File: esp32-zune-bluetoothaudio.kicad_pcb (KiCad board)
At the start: 2 copper layers, 36 parts, among them J1 Conn_01x06, J2 USB_C_Receptacle_USB2.0, J3 zune connector, Q1 MMBT3904, Q2 MMBT3904, Q3 MMBT3904, Q4 MMBT3904, U1 TPM, U2 ESP32-A1S, U3 AP1117-33

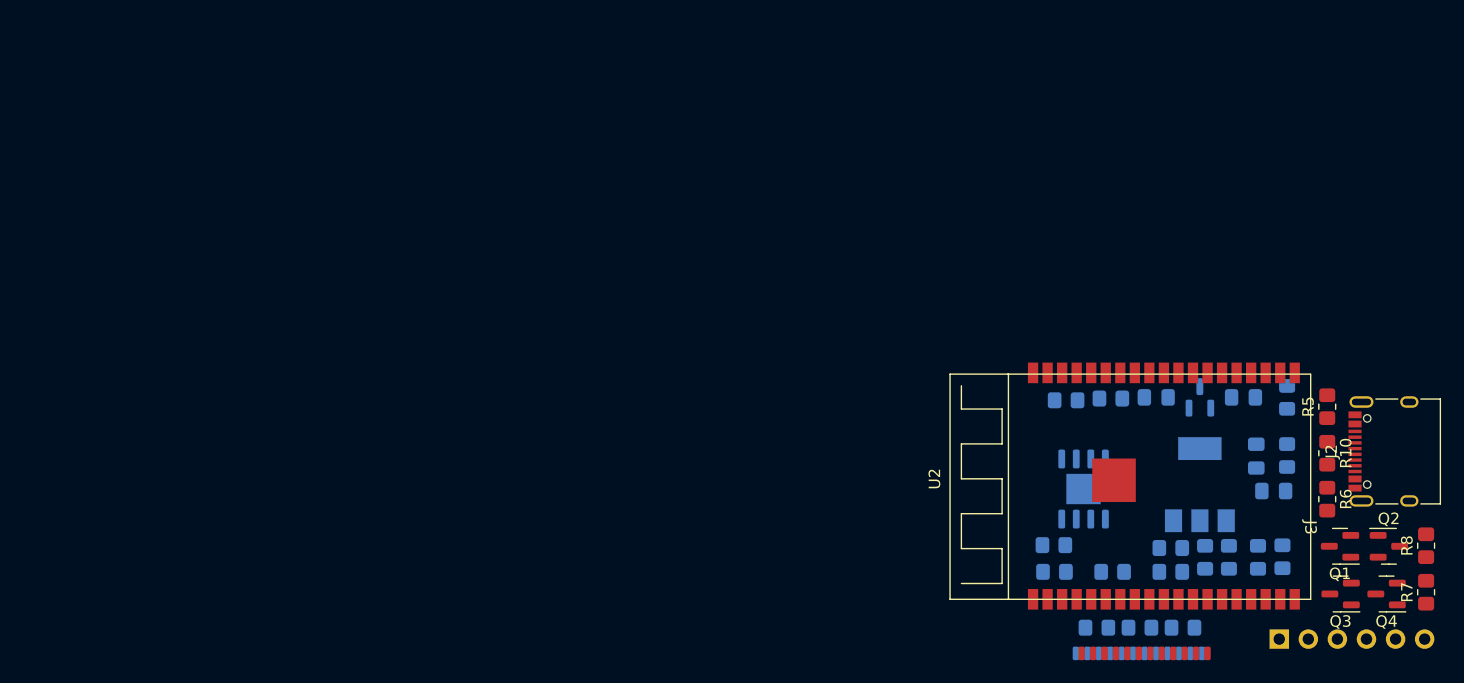
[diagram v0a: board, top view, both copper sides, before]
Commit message: layoutish
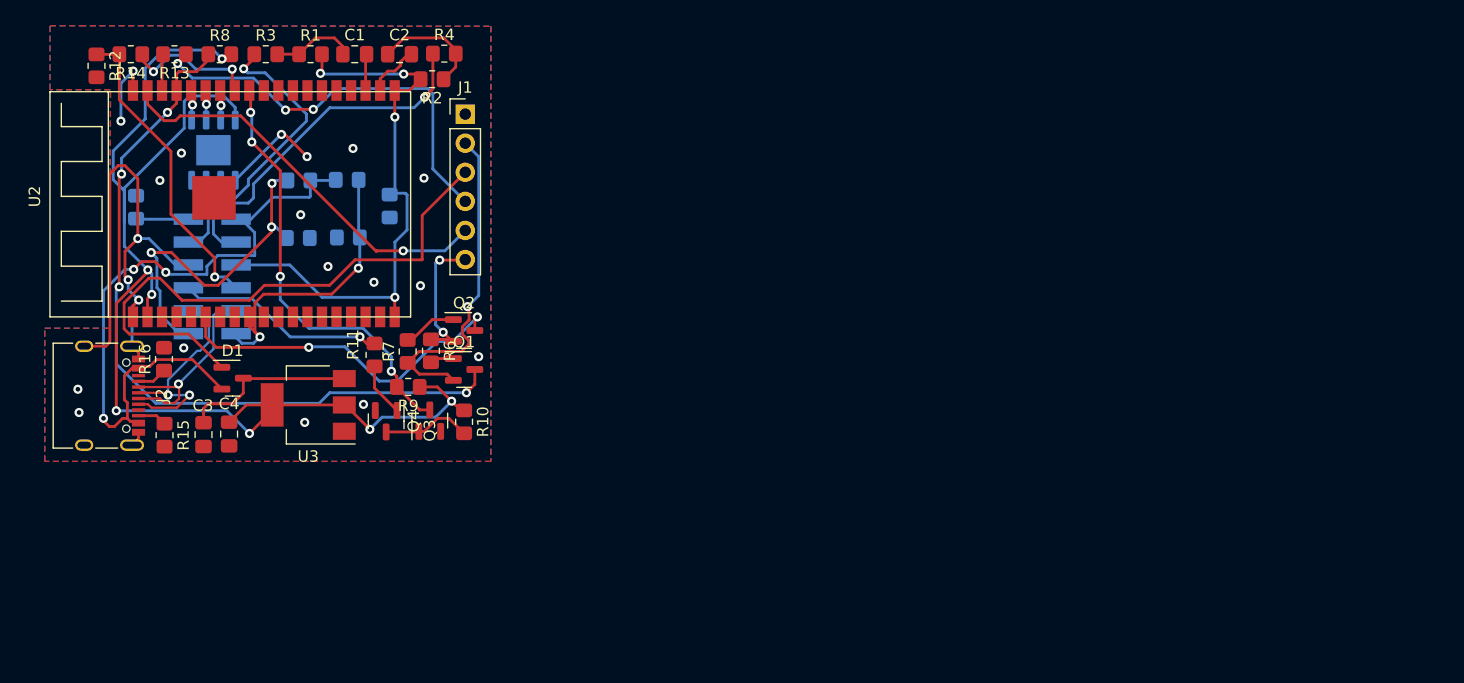
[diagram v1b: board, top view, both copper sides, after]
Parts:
- C1, C2, C3, C4, D1, R1, R11, R12, R13, R14, R15, R16, R2, R3, R4, R9, U3: moved to F.Cu
- J1: footprint Connector_PinSocket_2.54mm:PinSocket_1x06_P2.54mm_Horizontal -> Connector_PinHeader_2.54mm:PinHeader_1x06_P2.54mm_Vertical; moved to F.Cu
- J3: value zune connector -> Zune Passthrough; footprint ZuneConnector:zune-edge-connector -> Connector_PinHeader_2.00mm:PinHeader_2x06_P2.00mm_Vertical_SMD; moved to B.Cu
- R5: moved to B.Cu
- moved R8 113.8 mm to (120.1, 81.8), turned to 0 degrees
- moved J2 113.7 mm to (109.4, 111.6), turned to -90 degrees
- moved R14 104.7 mm to (112.4, 81.8)
- moved R16 98.5 mm to (115.3, 108.4), turned to 90 degrees
- moved R15 98.1 mm to (115.3, 115.1), turned to -90 degrees
- moved R12 93.2 mm to (109.4, 82.8), turned to -90 degrees
- moved R3 93.1 mm to (124.2, 81.8), turned to 0 degrees
- moved R1 91.5 mm to (128.1, 81.8), turned to 0 degrees
- moved R7 91.4 mm to (136.6, 107.7)
- moved R21 91.0 mm to (112.8, 95.1), turned to 90 degrees
- moved C1 88.9 mm to (131.9, 81.8)
- moved Q4 88.7 mm to (134.7, 113.8), turned to -90 degrees
- moved C4 88.7 mm to (121.0, 115.0), turned to -90 degrees
- moved J3 87.8 mm to (119.5, 101.2), turned to 180 degrees
- moved R2 85.2 mm to (138.7, 84.0), turned to 180 degrees
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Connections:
- J3 pad 10: unconnected-(J3-Pad10) -> usb D+
- J3 pad 11: unconnected-(J3-Pad11) -> auth_ctrl
- J3 pad 12: GNDA -> Net-(R17-Pad1)
- J3 pad 2: +5V -> Net-(R21-Pad1)
- J3 pad 3: +5V -> audio_r
- J3 pad 4: zune-rx -> audio_l
- J3 pad 5: zune-tx -> GNDA
- J3 pad 6: unconnected-(J3-Pad6) -> GND
- J3 pad 7: unconnected-(J3-Pad7) -> zune-rx
- J3 pad 8: unconnected-(J3-Pad8) -> zune-tx
- J3 pad 9: unconnected-(J3-Pad9) -> usb D-
- R17 pad 1: +5V -> Net-(R17-Pad1)
- R17 pad 2: Net-(J3-Pad19) -> +5V
- R18 pad 1: Net-(J3-Pad19) -> Net-(R17-Pad1)
- R20 pad 1: Net-(J3-Pad19) -> +5V
- R21 pad 1: GND -> Net-(R21-Pad1)
- R21 pad 2: Net-(J3-Pad17) -> GND
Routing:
- net +3.3V: track 0.00 -> 106.6 mm, vias 0 -> 7
- net EN: track 0.00 -> 65.5 mm, vias 0 -> 4
- net GND: track 0.00 -> 59.7 mm, vias 0 -> 21
- net +5V: track 0.00 -> 58.9 mm, vias 0 -> 3
- net +5C: track 0.00 -> 50.6 mm
- net GNDA: track 0.00 -> 49.0 mm, vias 0 -> 4
- net esp-rx: track 0.00 -> 37.5 mm, vias 0 -> 4
- net prg-rx: track 0.00 -> 36.6 mm, vias 0 -> 3
- net prg-tx: track 0.00 -> 35.4 mm, vias 0 -> 1
- net audio_r: track 0.00 -> 32.1 mm, vias 0 -> 1
- net esp_rst: track 0.00 -> 30.7 mm, vias 0 -> 2
- net rts: track 0.00 -> 29.6 mm, vias 0 -> 1
- net Net-(R17-Pad1): track 0.00 -> 29.2 mm, vias 0 -> 3
- net zune-rx: track 0.00 -> 27.2 mm, vias 0 -> 1
- net auth_ctrl: track 0.00 -> 25.8 mm, vias 0 -> 2
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- added copper zone on B.Cu, net GND
- added copper zone on F.Cu, net GND
